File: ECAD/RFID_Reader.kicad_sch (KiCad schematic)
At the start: 38 parts, among them P1 USB_C_Plug, SW1 SW_Push, Y2 27.12 MHz

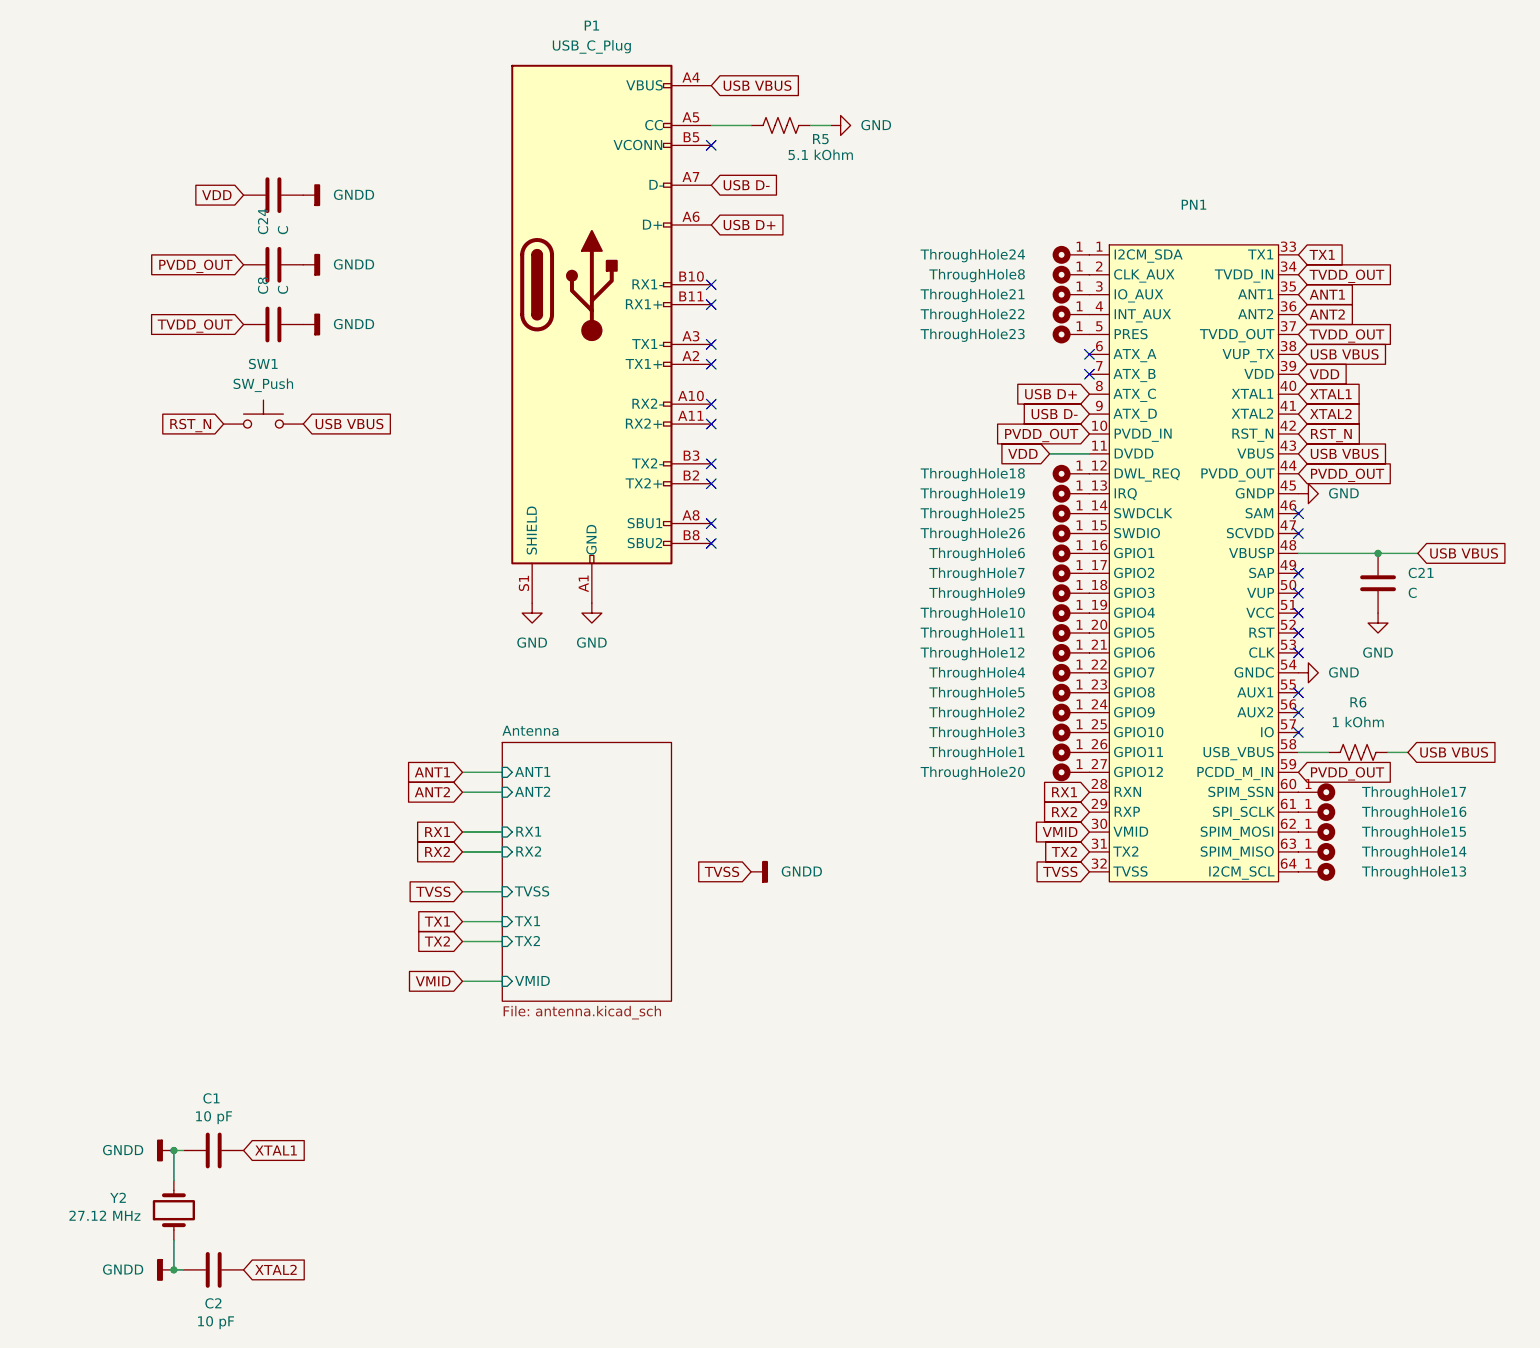
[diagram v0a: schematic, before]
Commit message: Updated schmatics
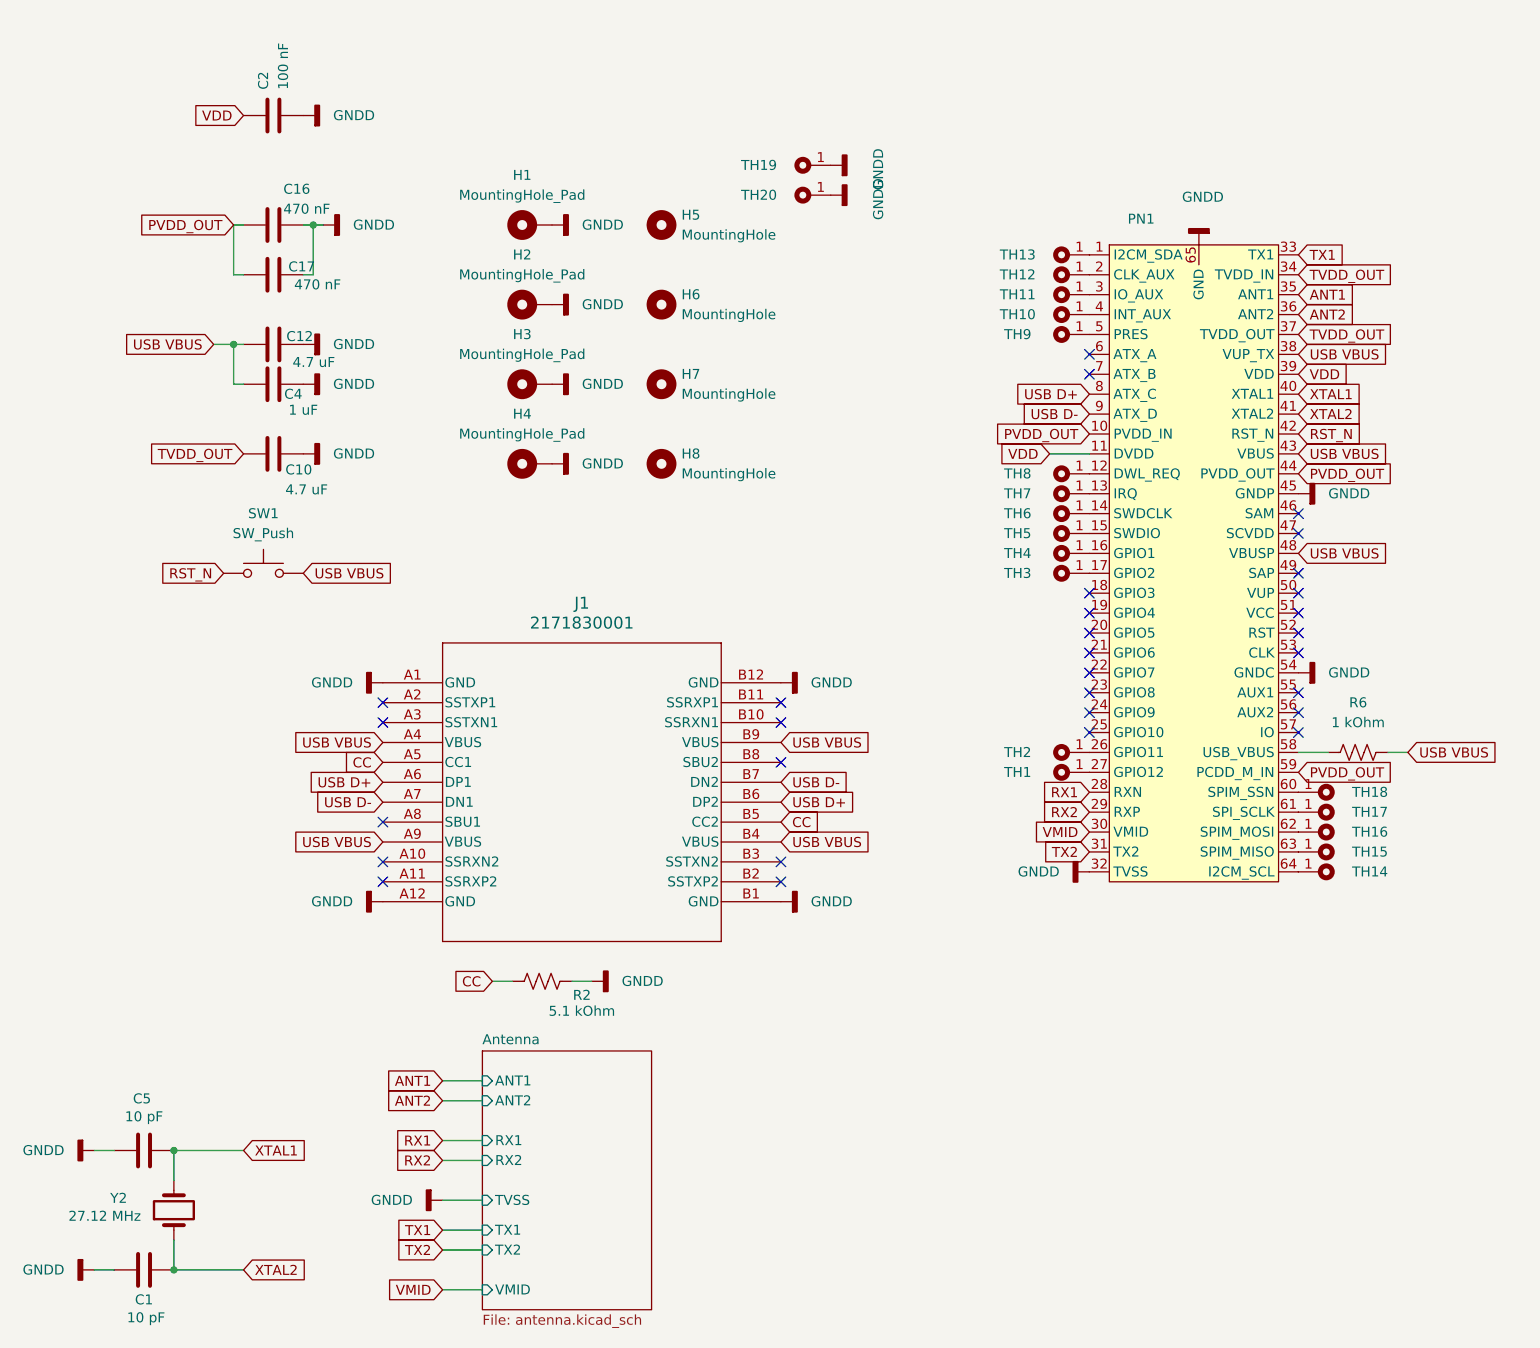
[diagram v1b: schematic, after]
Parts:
- removed C21, C22: C, Capacitor_SMD:C_01005_0402Metric, symbol Device:C
- removed P1: USB_C_Plug, Connector_USB:USB_C_Plug_JAE_DX07P024AJ1, symbol Connector:USB_C_Plug
- removed R5: 5.1 kOhm, Resistor_SMD:R_01005_0402Metric, symbol Device:R_US
- removed ThroughHole1, ThroughHole10, ThroughHole11, ThroughHole12, ThroughHole13, ThroughHole14, ThroughHole15, ThroughHole16, ThroughHole17, ThroughHole18, ThroughHole19, ThroughHole2, ThroughHole20, ThroughHole21, ThroughHole22, ThroughHole23, ThroughHole24, ThroughHole25, ThroughHole26, ThroughHole3, ThroughHole4, ThroughHole5, ThroughHole6, ThroughHole7, ThroughHole8, ThroughHole9: ~, Custom_Connector:TH22, symbol Custom_Connectors:ThroughHole
- added C12: 4.7 uF, Capacitor_SMD:C_0805_2012Metric, symbol Device:C
- added C17: 470 nF, Capacitor_SMD:C_0805_2012Metric, symbol Device:C
- added C4: 1 uF, Capacitor_SMD:C_0805_2012Metric, symbol Device:C
- added C5: 10 pF, Capacitor_SMD:C_0805_2012Metric, symbol Device:C
- added H1, H2, H3, H4: MountingHole_Pad, MountingHole:MountingHole_3.5mm_Pad, symbol Mechanical:MountingHole_Pad
- added H5, H6, H7, H8: MountingHole, Custom_Connector:MountingHole_60mil, symbol Mechanical:MountingHole
- added J1: 2171830001, footprints:CONN_2171830001_MOL, symbol 2026-03-16_18-54-40:2171830001
- added R2: 5.1 kOhm, Resistor_SMD:R_0805_2012Metric, symbol Device:R_US
- added TH1, TH10, TH11, TH12, TH13, TH14, TH15, TH16, TH17, TH18, TH19, TH2, TH20, TH3, TH4, TH5, TH6, TH7, TH8, TH9: ~, Custom_Connector:TH22, symbol Custom_Connectors:TH
- C1: footprint Capacitor_SMD:C_01005_0402Metric -> Capacitor_SMD:C_0805_2012Metric
- C10: renamed from C8; value C -> 4.7 uF; footprint Capacitor_SMD:C_01005_0402Metric -> Capacitor_SMD:C_0805_2012Metric
- C16: renamed from C24; value C -> 470 nF; footprint Capacitor_SMD:C_01005_0402Metric -> Capacitor_SMD:C_0805_2012Metric
- C2: value 10 pF -> 100 nF; footprint Capacitor_SMD:C_01005_0402Metric -> Capacitor_SMD:C_0805_2012Metric
- R6: footprint Resistor_SMD:R_01005_0402Metric -> Resistor_SMD:R_0805_2012Metric
- SW1: footprint Button_Switch_SMD:SW_MEC_5GSH9 -> Button_Switch_THT:SW_PUSH_6mm
- Y2: footprint Oscillator:Oscillator_DIP-8 -> Crystal:Crystal_SMD_0603-2Pin_6.0x3.5mm_HandSoldering
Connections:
- net GND is gone; now on net GNDD: PN1.45 (GNDP), PN1.54 (GNDC)
- net GNDD: now also PN1.65 (GND), C12.2, C17.2, C4.1, C5.2, H1.1, H2.1, H3.1, H4.1, J1.A1 (GND), J1.A12 (GND), J1.B1 (GND), J1.B12 (GND), R2.2, TH19.1, TH20.1; no longer Y2.1, Y2.2
- net PVDD_OUT: now also C17.1
- net USB D+: now also J1.A6 (DP1), J1.B6 (DP2)
- net USB D-: now also J1.A7 (DN1), J1.B7 (DN2)
- net USB VBUS: now also C12.1, C4.2, J1.A4 (VBUS), J1.A9 (VBUS), J1.B4 (VBUS), J1.B9 (VBUS)
- net VDD: now also C2.1
- net XTAL1: now also Y2.2, C5.1; no longer C1.1
- net XTAL2: now also C1.1, Y2.1; no longer C2.1
- net at PN1.2 (CLK_AUX): now also TH12.1
- net at PN1.13 (IRQ): now also TH7.1
- net at PN1.60 (SPIM_SSN): now also TH18.1
- net at PN1.4 (INT_AUX): now also TH10.1
- net at PN1.26 (GPIO11): now also TH2.1
- net at PN1.27 (GPIO12): now also TH1.1
- net at PN1.1 (I2CM_SDA): now also TH13.1
- net at PN1.63 (SPIM_MISO): now also TH15.1
- net at PN1.3 (IO_AUX): now also TH11.1
- net at PN1.15 (SWDIO): now also TH5.1
- net at PN1.5 (PRES): now also TH9.1
- net at PN1.62 (SPIM_MOSI): now also TH16.1
- net at PN1.17 (GPIO2): now also TH3.1
- net at PN1.16 (GPIO1): now also TH4.1
- net at PN1.12 (DWL_REQ): now also TH8.1
- net at PN1.14 (SWDCLK): now also TH6.1
- net at PN1.61 (SPI_SCLK): now also TH17.1
- net at PN1.64 (I2CM_SCL): now also TH14.1
- new net CC: J1.A5 (CC1), J1.B5 (CC2), R2.1
- no-connect marks 23 -> 30
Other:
- moved on the sheet: C10, C16, SW1
